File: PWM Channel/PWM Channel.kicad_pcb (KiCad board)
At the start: 2 copper layers, 24 parts, among them J101 Conn_01x05_Male, U201 NE555P, U302 4040, U304 7485, U305 7485, U306 7485, U401 74HCT595, U402 74HCT595

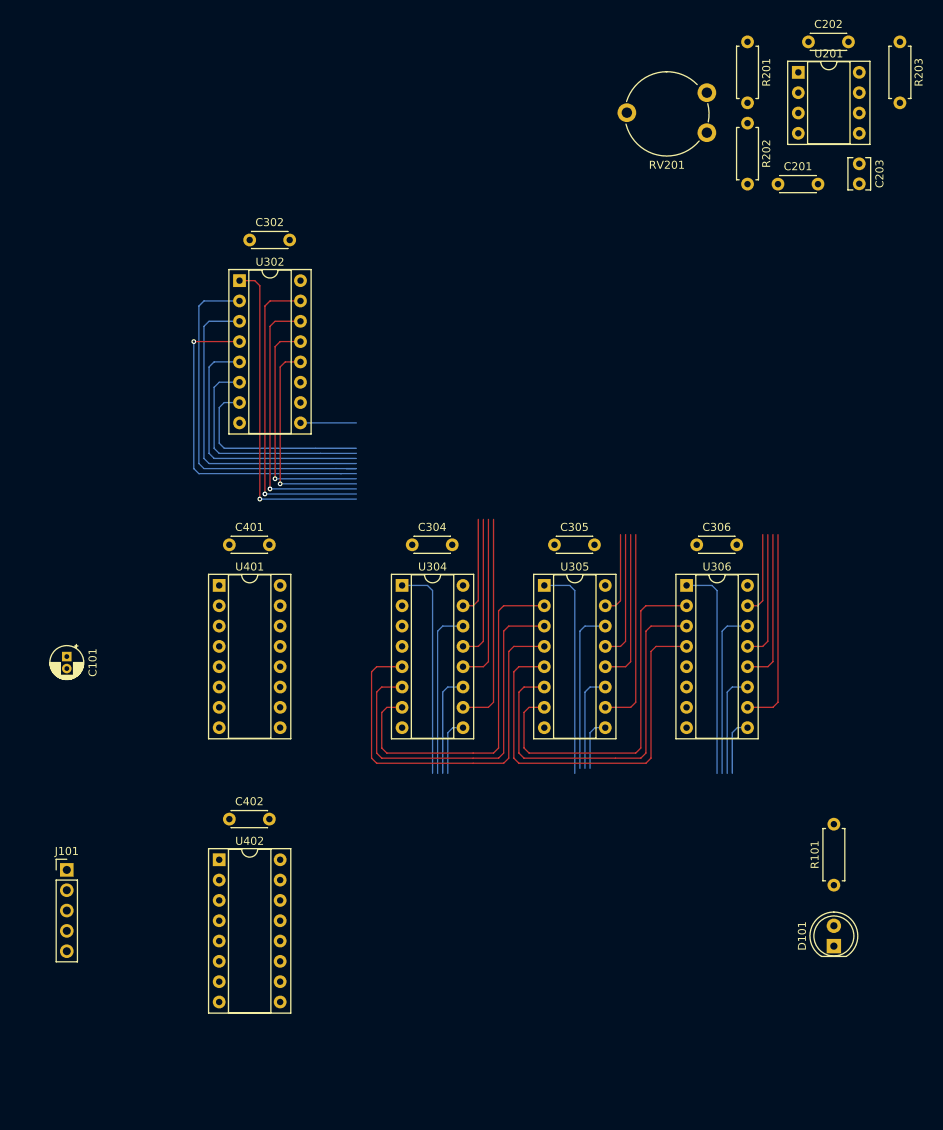
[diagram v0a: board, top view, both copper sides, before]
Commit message: Preliminary routing
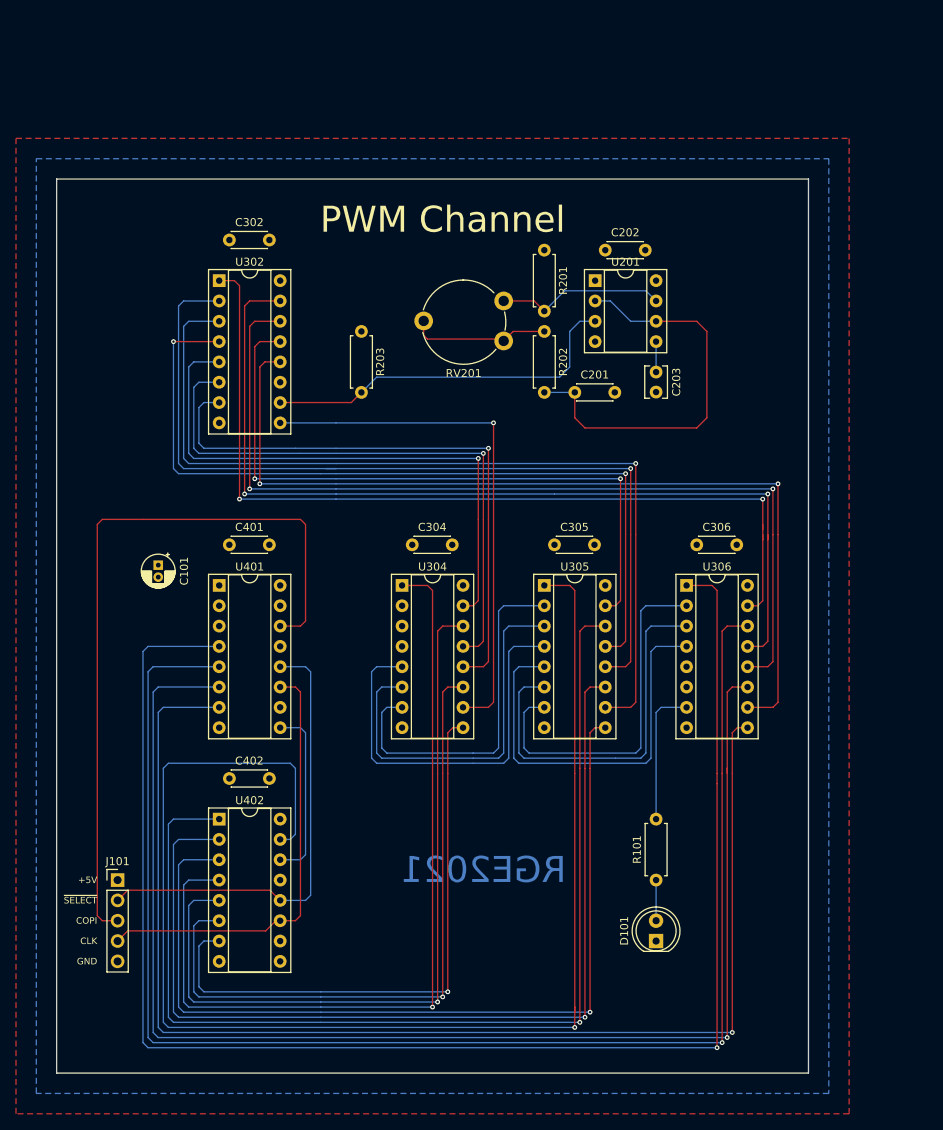
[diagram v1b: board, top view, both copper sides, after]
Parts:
- R201, R202: value 33 -> 4.7
- moved R203 76.4 mm to (43.2, -8.89)
- moved C201 36.4 mm to (69.8, -1.27)
- moved C202 36.4 mm to (73.7, -19.1)
- moved RV201 36.4 mm to (61.0, -12.7)
- moved U201 36.4 mm to (72.4, -15.2)
- moved C203 36.4 mm to (80.0, -3.81)
- moved R201 36.4 mm to (66.0, -19.1)
- moved R202 36.4 mm to (66.0, -8.89)
- moved D101 22.2 mm to (80.0, 67.3)
- moved R101 22.2 mm to (80.0, 59.7)
- moved C101 16.2 mm to (17.8, 20.3)
- moved J101 6.48 mm to (12.7, 59.7)
- moved C402 5.08 mm to (26.7, 47.0)
- moved U402 5.08 mm to (25.4, 52.1)
- moved U302 2.54 mm to (25.4, -15.2)
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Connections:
- J101 pad 2: /SPI Input/CLK -> /SPI Input/~SELECT
- J101 pad 4: /SPI Input/~SELECT -> /SPI Input/CLK
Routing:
- net /PWM/B11: track 26.9 -> 191.9 mm, vias 0 -> 1
- net /PWM/B10: track 21.2 -> 181.8 mm, vias 0 -> 1
- net /PWM/B09: track 13.0 -> 169.7 mm, vias 0 -> 1
- net /PWM/B08: track 7.25 -> 158.9 mm, vias 0 -> 1
- net /PWM/B07: track 26.9 -> 170.2 mm, vias 0 -> 1
- net /PWM/B06: track 20.6 -> 134.8 mm, vias 0 -> 1
- net /PWM/B05: track 12.3 -> 122.1 mm, vias 0 -> 1
- net /PWM/B04: track 6.61 -> 111.9 mm, vias 0 -> 1
- net /SPI Input/COPI: track 0.00 -> 93.8 mm
- net /PWM/B03: track 26.9 -> 106.8 mm, vias 0 -> 1
- net /PWM/B02: track 21.2 -> 96.7 mm, vias 0 -> 1
- net /PWM/B01: track 13.0 -> 84.0 mm, vias 0 -> 1
- net /PWM/B00: track 7.25 -> 73.8 mm, vias 0 -> 1
- net /PWM/A08: track 52.0 -> 113.6 mm, vias 1 -> 2
- net /PWM/A09: track 54.5 -> 114.8 mm, vias 1 -> 2
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- added copper zone on B.Cu, net +5V
- added copper zone on F.Cu, net GND
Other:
- board outline added: 94 x 111.8 mm
- board text added: "+5V"
- board text added: "CLK"
- board text added: "COPI"
- board text added: "GND"
- board text added: "PWM Channel"
- board text added: "RGE2021"
- board text added: "~SELECT"
